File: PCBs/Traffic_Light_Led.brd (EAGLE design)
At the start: 33 x 28 mm, 10 parts

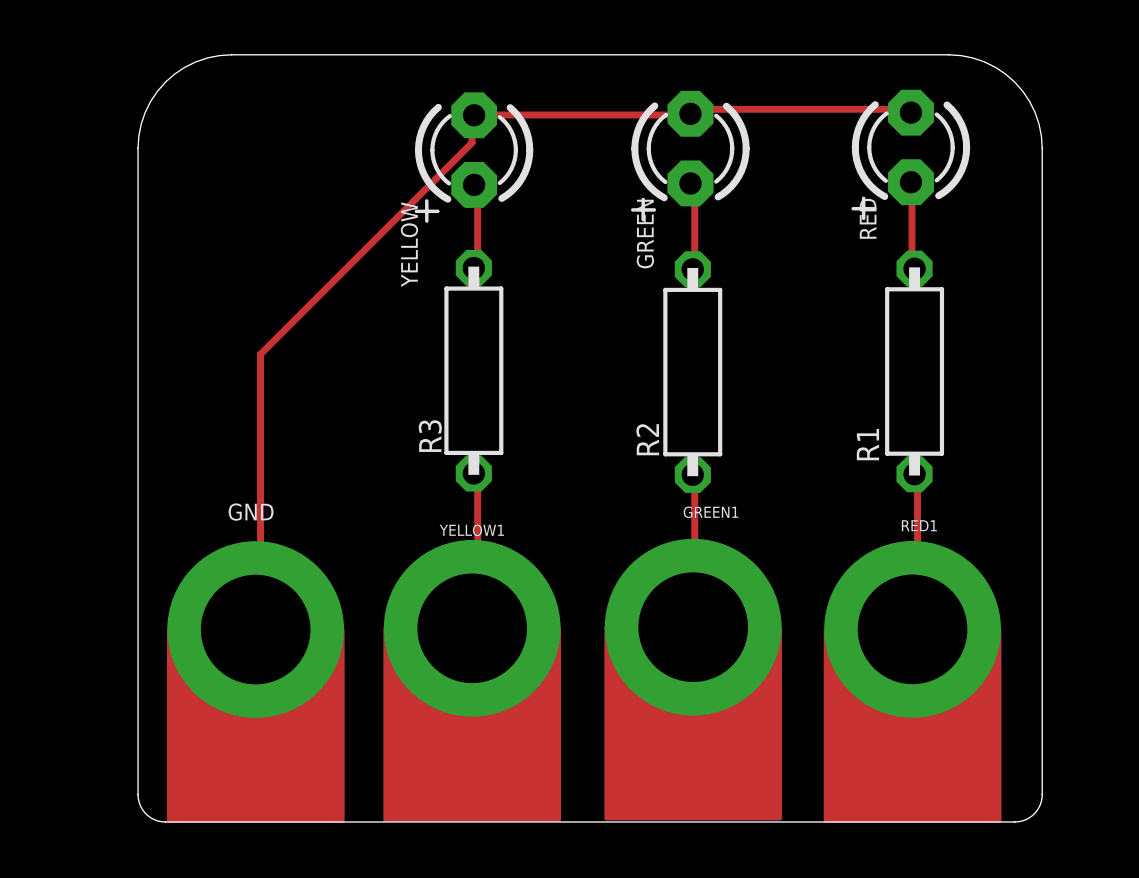
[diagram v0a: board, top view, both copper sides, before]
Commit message: New Update
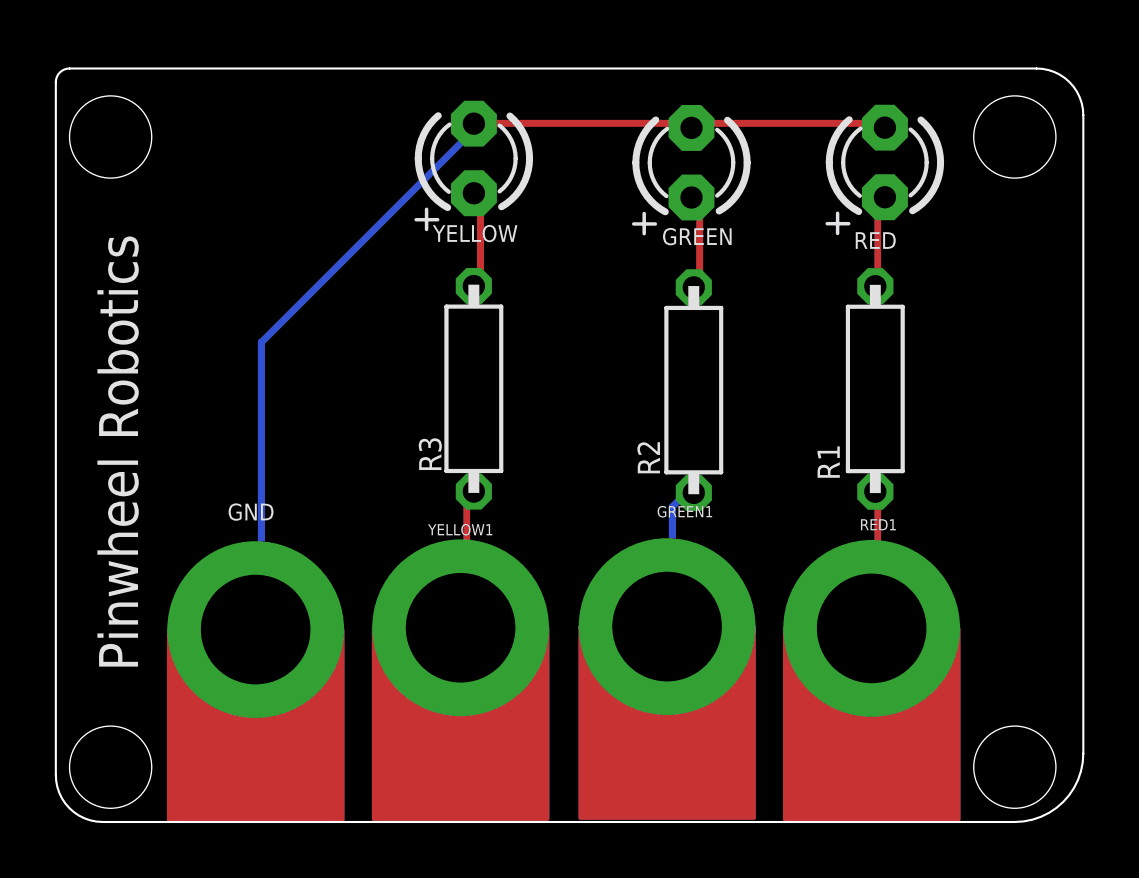
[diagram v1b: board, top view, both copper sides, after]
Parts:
- moved R1 1.57 mm to (26.9, 15.8)
- moved RED1 1.49 mm to (26.8, 7.07)
- moved RED 1.10 mm to (27.3, 24.1)
- moved GREEN1 0.95 mm to (19.3, 7.13)
- moved R2 0.66 mm to (20.3, 15.8)
- moved R3 0.66 mm to (12.3, 15.8)
- moved GREEN 0.51 mm to (20.2, 24.1)
- moved YELLOW1 0.42 mm to (11.8, 7.09)
- moved YELLOW 0.31 mm to (12.3, 24.2)
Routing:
- net GND: track 38.2 -> 36.8 mm
- net N$1: track 5.83 -> 5.10 mm
- net N$2: track 5.87 -> 5.23 mm
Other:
- board size 33 x 28 mm -> 37.5 x 27.5 mm
- board text added: "Pinwheel Robotics"
- board text added: "care@pinwheel.in"
